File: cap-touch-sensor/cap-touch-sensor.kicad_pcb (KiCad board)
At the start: 2 copper layers, 15 x 15 mm, 10 parts, among them U1 TTP223-BA6

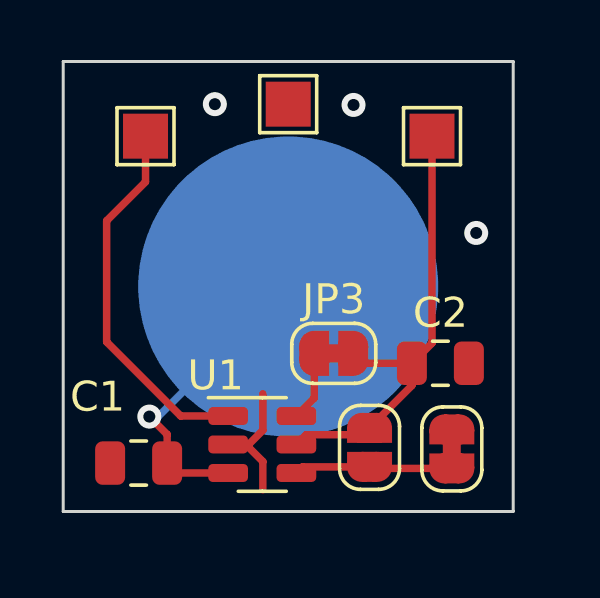
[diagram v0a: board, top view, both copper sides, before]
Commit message: Update CAD files and gitignore
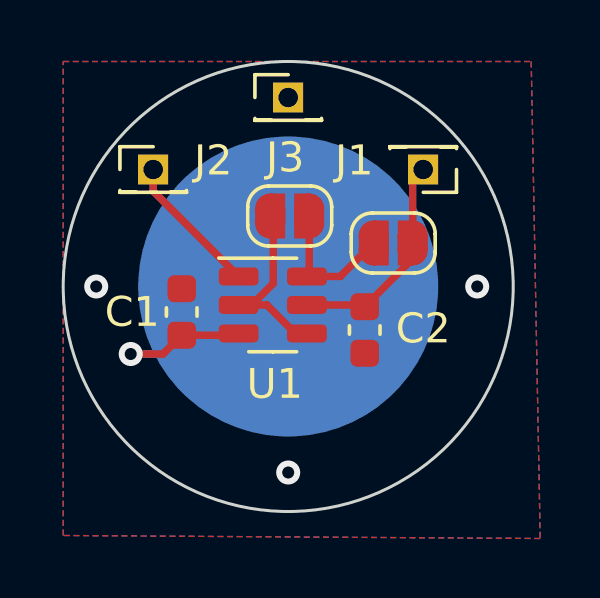
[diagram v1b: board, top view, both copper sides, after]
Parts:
- removed JP3: SolderJumper_2_Bridged, Jumper:SolderJumper-2_P1.3mm_Bridged_RoundedPad1.0x1.5mm
- removed TP1: Vcc, TestPoint:TestPoint_Pad_1.5x1.5mm
- removed TP2: TOGGLE, TestPoint:TestPoint_Pad_1.5x1.5mm
- removed TP3: GND, TestPoint:TestPoint_Pad_1.5x1.5mm
- added J1: VBAT, Connector_PinHeader_1.27mm:PinHeader_1x01_P1.27mm_Vertical, F.Cu at (12.0, 3.60)
- added J2: TOG, Connector_PinHeader_1.27mm:PinHeader_1x01_P1.27mm_Vertical, F.Cu at (3.00, 3.60)
- added J3: GND, Connector_PinHeader_1.27mm:PinHeader_1x01_P1.27mm_Vertical, F.Cu at (7.50, 1.20)
- C1, C2: footprint Capacitor_SMD:C_0805_2012Metric -> Capacitor_SMD:C_0603_1608Metric
- JP2: value SolderJumper_2_Bridged -> SolderJumper_2_Open; footprint Jumper:SolderJumper-2_P1.3mm_Bridged_RoundedPad1.0x1.5mm -> Jumper:SolderJumper-2_P1.3mm_Open_RoundedPad1.0x1.5mm
- moved JP2 9.46 mm to (7.55, 5.15), turned to 0 degrees
- moved JP1 6.86 mm to (11.0, 6.05), turned to 0 degrees
- moved C1 5.24 mm to (3.95, 8.35), turned to 90 degrees
- moved U1 4.66 mm to (6.98, 8.12)
- moved C2 2.76 mm to (10.1, 8.95), turned to -90 degrees
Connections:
- U1 pad 4: Net-(JP1-A) -> GND
- U1 pad 6: Net-(JP3-A) -> Net-(JP1-A)
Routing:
- net VBAT: track 15.5 -> 7.33 mm
- net TOGGLE: track 12.5 -> 4.75 mm
- net Net-(JP3-A): track 2.33 -> 0.00 mm
- net GND: track 4.91 -> 6.41 mm
- net Net-(JP1-A): track 5.29 -> 4.74 mm
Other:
- outline, holes or cut-outs redrawn
